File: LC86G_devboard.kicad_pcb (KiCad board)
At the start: 4 copper layers, 40 x 40 mm, 14 parts, among them J1 Conn_01x09_Pin, J2 U.FL-R-SMT_10_, Q1 DTC143Z, Q2 DTC143Z, Q3 AO3415, U1 LC86G

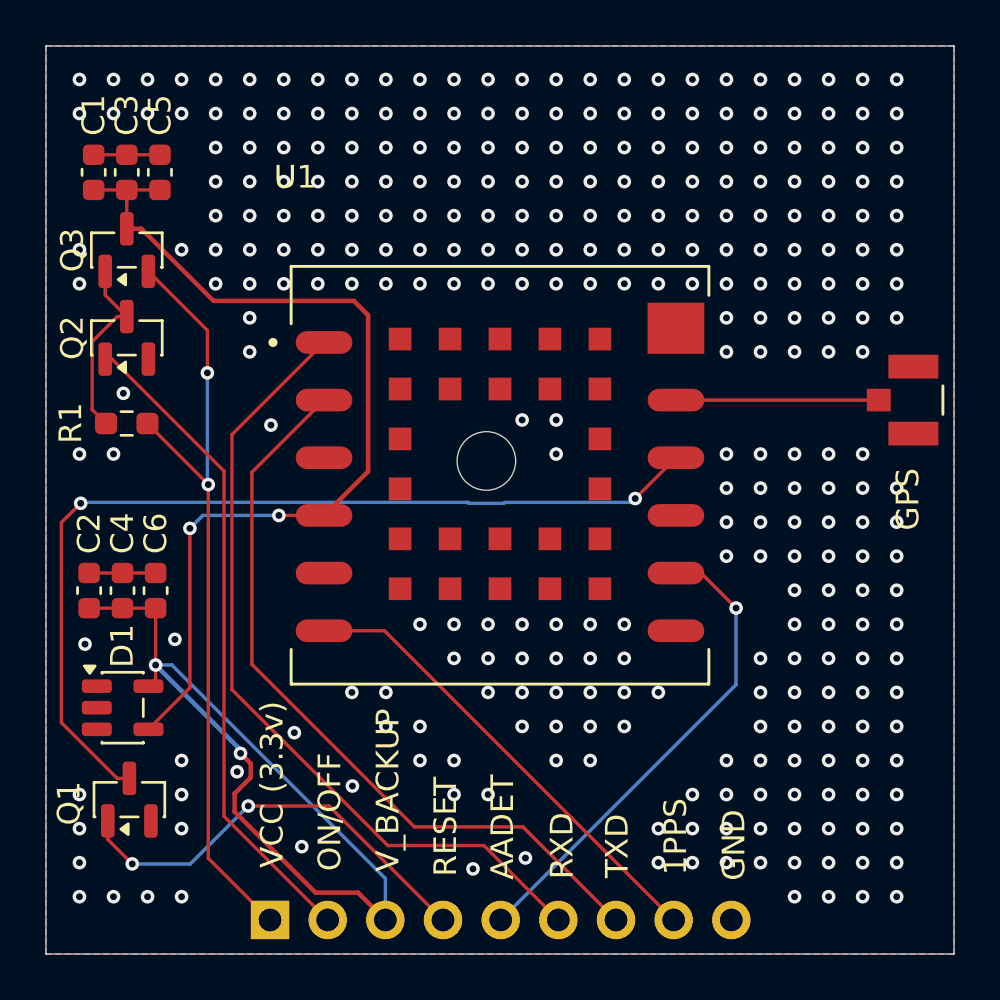
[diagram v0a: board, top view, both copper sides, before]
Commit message: carga final
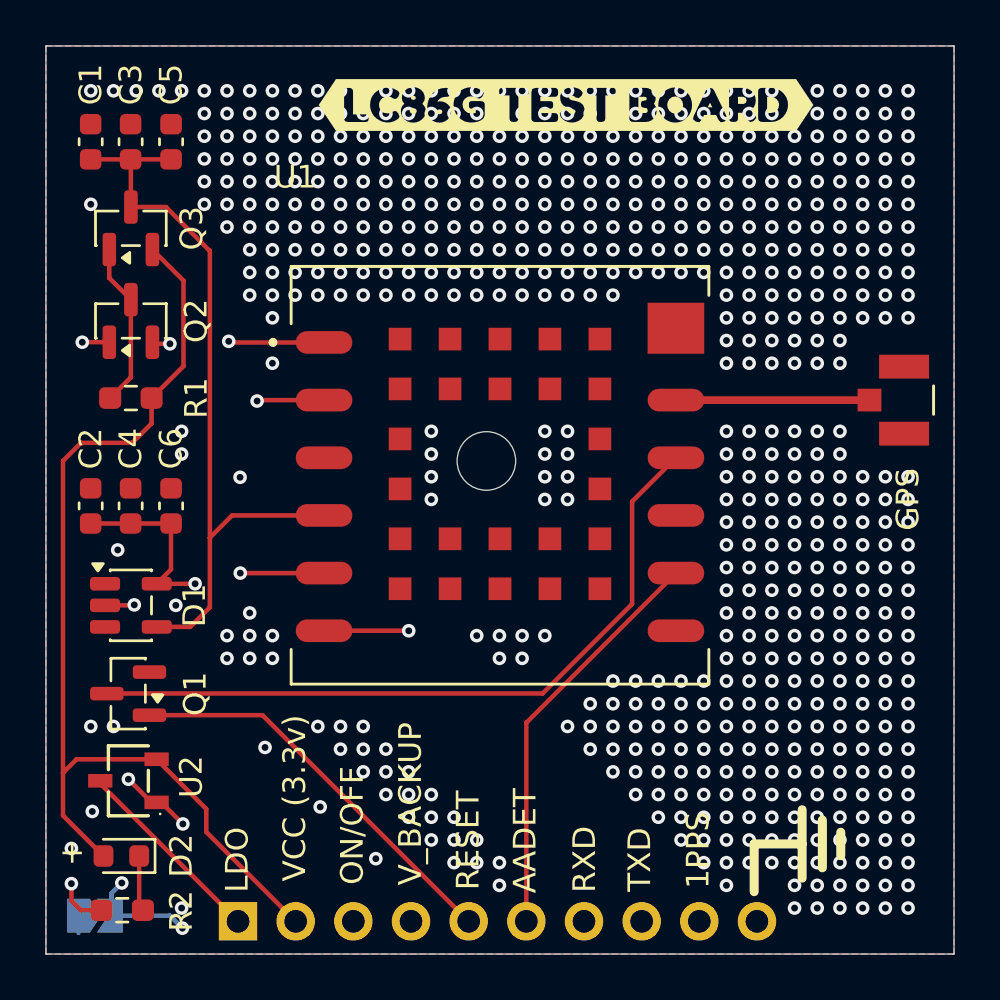
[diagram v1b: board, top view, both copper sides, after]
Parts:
- removed J1: Conn_01x09_Pin, Connector_PinHeader_2.54mm:PinHeader_1x09_P2.54mm_Vertical
- added D2: LED_Small, LED_SMD:LED_0603_1608Metric, F.Cu at (146.4, 106.2)
- added J3: Conn_01x10_Pin, Connector_PinHeader_2.54mm:PinHeader_1x10_P2.54mm_Vertical, B.Cu at (151.5, 109.1)
- added Power indicator: SolderJumper_2_Open, Jumper:SolderJumper-2_P1.3mm_Open_TrianglePad1.0x1.5mm, B.Cu at (145.2, 108.8)
- added R2: 4.7k, Resistor_SMD:R_0603_1608Metric_Pad0.98x0.95mm_HandSolder, F.Cu at (146.4, 108.6)
- added U2: XC6206P332MR, EasyEDA:SOT-23-3_L2.9-W1.6-P1.90-LS2.8-BR, F.Cu at (146.7, 102.9)
- added kibuzzard-6A1C8FBC: G***, kibuzzard-6A1C8FBC, F.Cu at (166.0, 73.1)
- moved Q1 4.67 mm to (146.7, 99.0), turned to 180 degrees
- moved D1 4.52 mm to (146.8, 95.2)
- moved C6 3.79 mm to (148.6, 90.8)
- moved C4 3.75 mm to (146.8, 90.8)
- moved C2 3.73 mm to (145.0, 90.8)
- moved C5 1.43 mm to (148.6, 74.7)
- moved C3 1.36 mm to (146.8, 74.7)
- moved C1 1.35 mm to (145.0, 74.7)
- moved R1 1.13 mm to (146.8, 86.0)
- moved Q3 0.97 mm to (146.8, 78.5)
- moved Q2 0.77 mm to (146.8, 82.6)
- moved J2 0.41 mm to (180.8, 86.1)
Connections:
- C2 pad 1: /V_BCKP -> /LC86G.V_BCKP
- C4 pad 1: /V_BCKP -> /LC86G.V_BCKP
- C6 pad 1: /V_BCKP -> /LC86G.V_BCKP
- D1 pad 5: /V_BCKP -> /LC86G.V_BCKP
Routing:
- net /V_BCKP: track 39.5 -> 0.00 mm, vias 2 -> 0
- net /LC86G.V_BCKP: track 0.00 -> 32.8 mm, vias 0 -> 2
- net /VCC: track 34.6 -> 45.6 mm, vias 2 -> 0
- net /LC86G.RESET: track 41.2 -> 32.0 mm, vias 2 -> 0
- net /LDO: track 0.00 -> 8.70 mm
- net /LC86G.VCC: track 42.3 -> 33.8 mm, vias 2 -> 0
- net Net-(JP1-A): track 0.00 -> 4.54 mm, vias 0 -> 1
- net GND: track 5.85 -> 9.54 mm, vias 308 -> 630
- net /LC86G.AADET: track 21.3 -> 18.1 mm, vias 1 -> 0
- net /ON/OFF: track 28.9 -> 31.7 mm, vias 0 -> 1
- net Net-(D2-K): track 0.00 -> 2.46 mm
- net /GPIO.RESET: track 19.2 -> 17.8 mm, vias 2 -> 0
- net /LC86G.1PPS: track 20.7 -> 21.8 mm, vias 0 -> 1
- net Net-(Q2-C): track 8.36 -> 7.31 mm
- net /LC86G.RXD: track 35.6 -> 36.4 mm, vias 0 -> 1
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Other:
- board text added: "+"
- board text added: "LDO"
- board text removed: "GND"

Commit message: aa
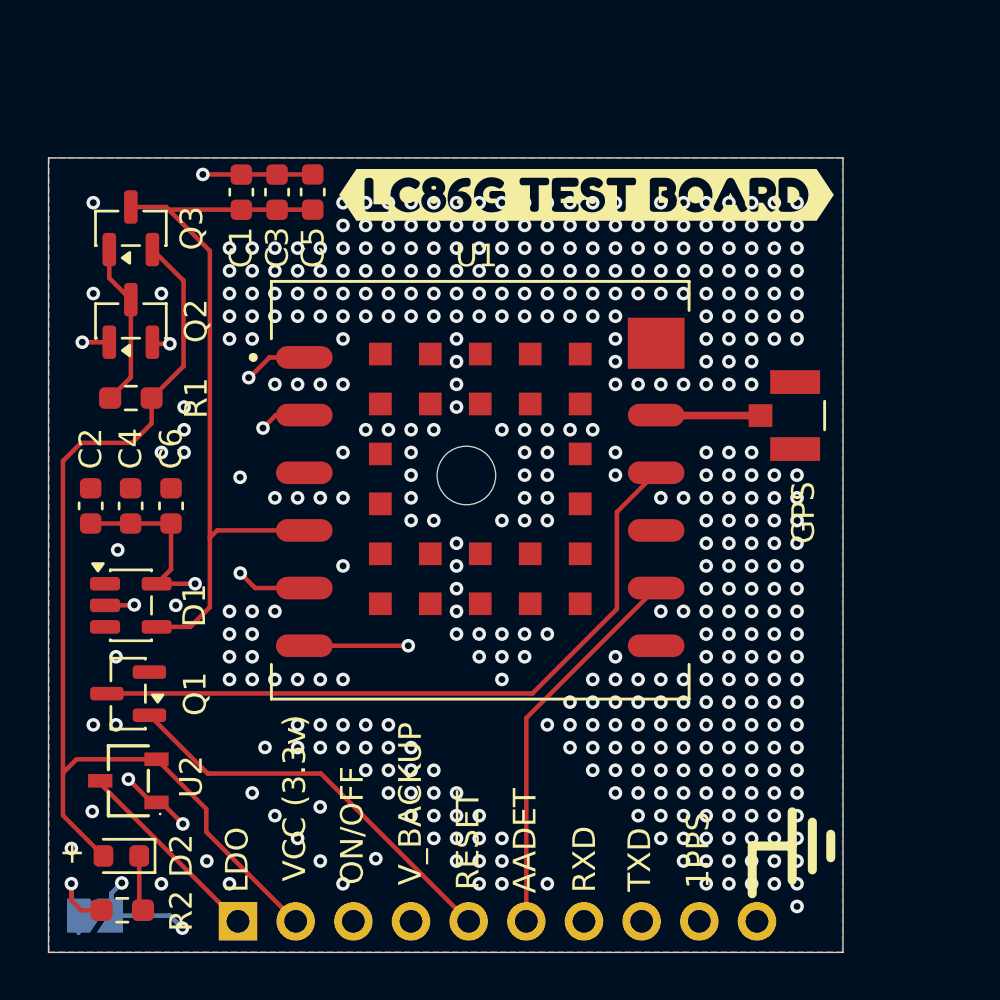
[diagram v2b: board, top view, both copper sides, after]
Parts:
- moved C1 7.00 mm to (151.7, 77.0)
- moved C3 6.82 mm to (153.2, 77.0)
- moved C5 6.62 mm to (154.8, 76.9)
- moved J2 4.85 mm to (176.1, 86.8)
- moved kibuzzard-6A1C8FBC 4.06 mm to (166.9, 77.1)
- moved U1 1.09 mm to (162.2, 90.1)
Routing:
- net GND: track 9.54 -> 14.4 mm, vias 630 -> 437
- net /LC86G.EX_ANT: track 8.52 -> 4.79 mm
- net /LC86G.RXD: track 36.4 -> 33.7 mm
- net /LC86G.TXD: track 32.9 -> 31.1 mm
- net /LC86G.RESET: track 32.0 -> 30.7 mm
- net /LC86G.AADET: track 18.1 -> 17.0 mm
- net /LC86G.1PPS: track 21.8 -> 22.4 mm
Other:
- board size 40 x 40 mm -> 35 x 35 mm
